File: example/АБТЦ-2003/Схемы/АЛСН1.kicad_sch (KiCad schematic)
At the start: 44 parts

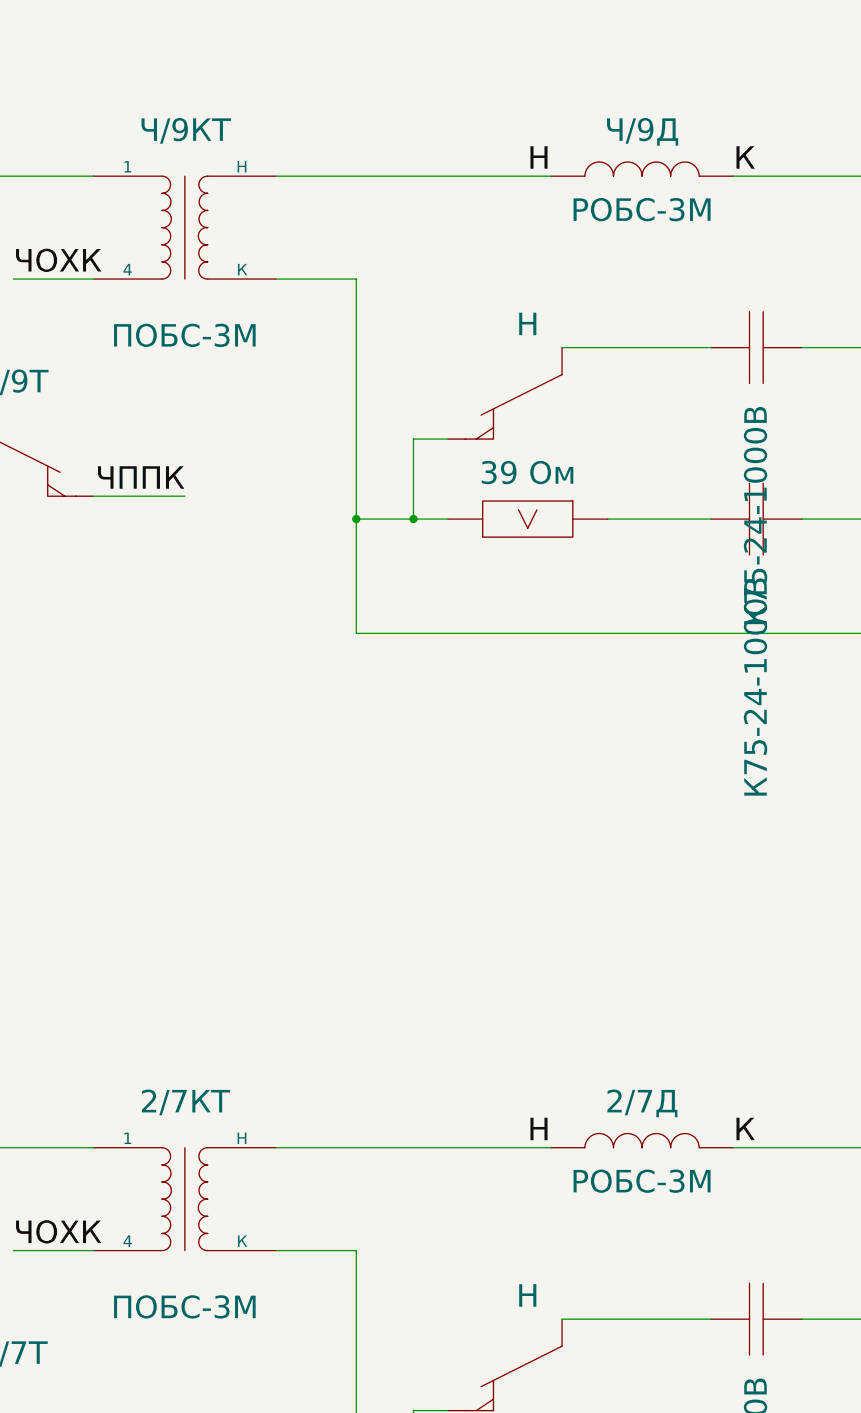
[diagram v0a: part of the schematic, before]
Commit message: Обновление примера
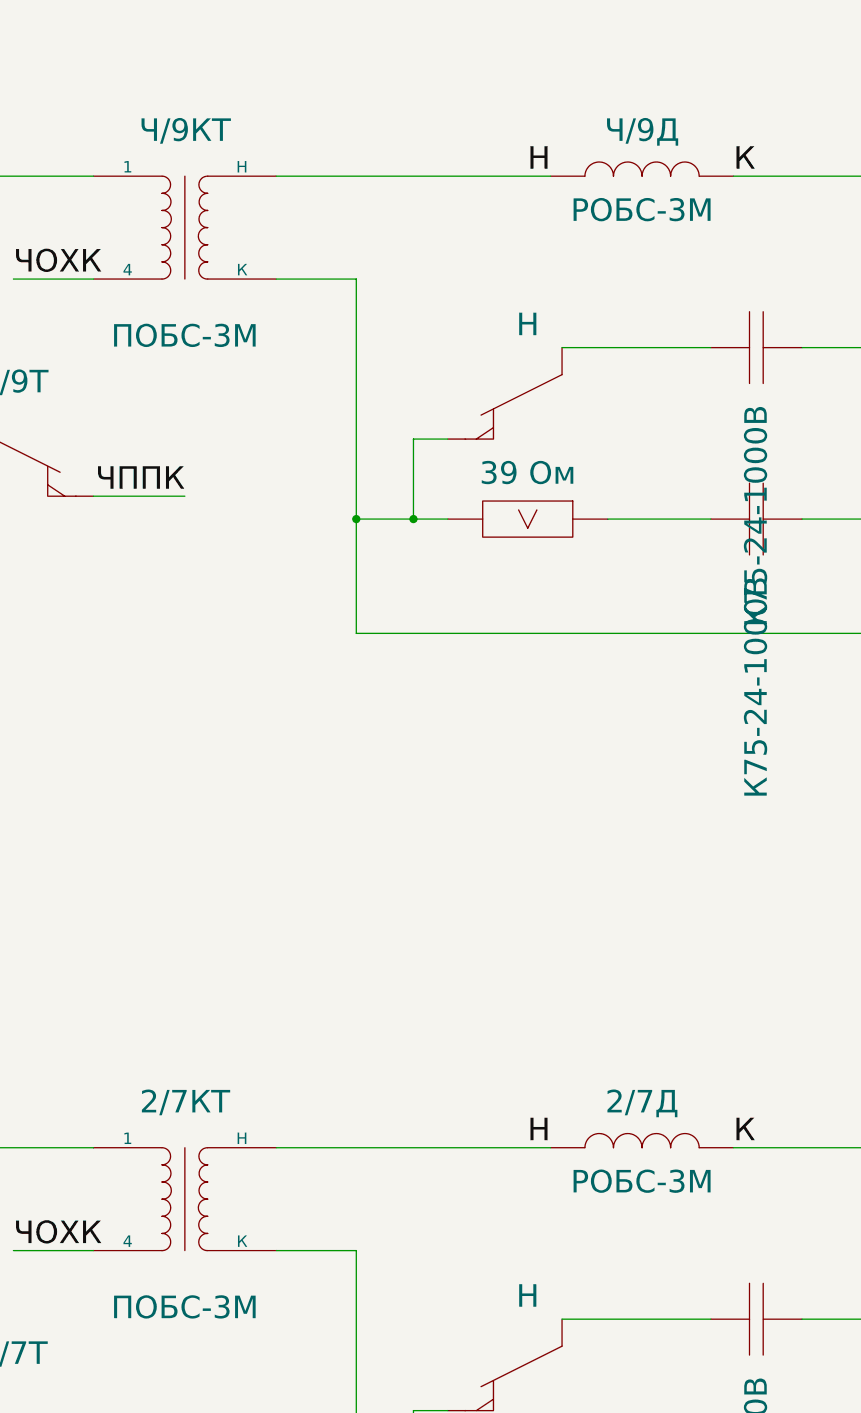
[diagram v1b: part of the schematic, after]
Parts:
- Н1, Н11, Н111, Н1111, Н11111, Н111111, Н1112, Н11121, Н111211, Н1113, Н11131, Н111311, Н1114, Н11141, Н1115, Н112: symbol SCB_Relay:Контакт_нейтрального_якоря -> SCB_Legacy:Контакт_нейтрального_якоря_бн
- Н111111, Н1111111: symbol SCB_Relay:Контакт_нейтрального_якоря_НЗ -> SCB_Legacy:Контакт_нейтрального_якоря_НЗ_бн
